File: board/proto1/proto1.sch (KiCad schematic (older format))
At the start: 86 parts, among them J1 Micro_SD_Card_Det, J10 GND, J11 J11, J11A1 J11A, J12 VBatt, J13 VBattSw, J14 LCD, J15 3.3V Out, J2 LED_DOUT, J3 Expansion, J4 +3.3V, J5 J5, J5A1 J5A, J6 J6, J6A1 J6A, J7 J7, J7A1 J7A, J8 J8, J8A1 J8A, J9 J9, J9A1 J9A, SW1 UP, SW2 LEFT, SW3 RIGHT, SW4 DOWN, SW5 ACTION, SW6 TILT, U1 MCP1603T-330I/OS

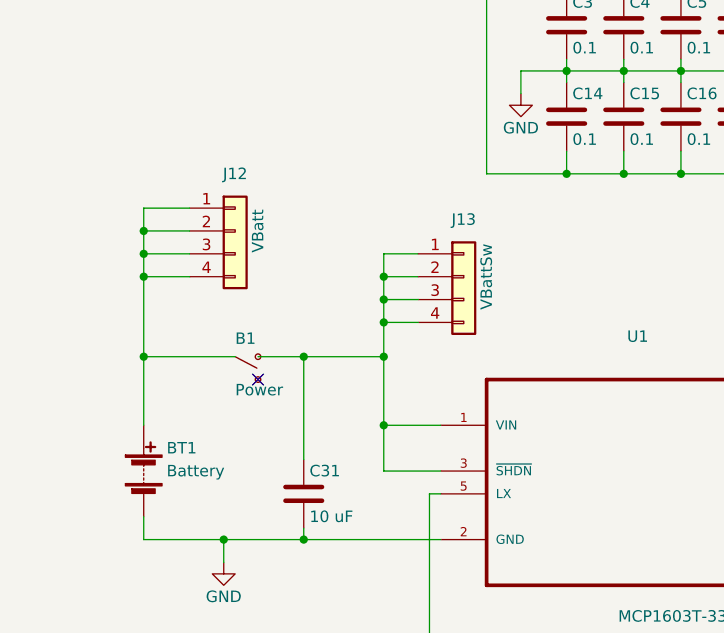
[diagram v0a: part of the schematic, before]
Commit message: layout maybe finished
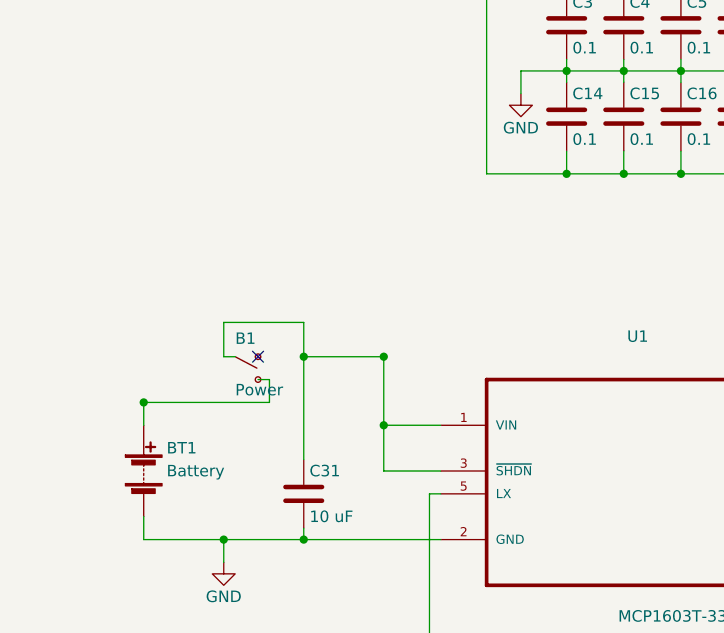
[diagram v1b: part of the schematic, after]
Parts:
- removed J12: VBatt, Pin_Headers:Pin_Header_Straight_1x04_Pitch2.54mm, symbol Conn_01x04
- removed J13: VBattSw, Pin_Headers:Pin_Header_Straight_1x04_Pitch2.54mm, symbol Conn_01x04
- J1: footprint 1140084168:1140084168 -> sdcard:newsdcard
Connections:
- net at B1.1 (B): now also BT1.1 (+)
- net at B1.2 (COM): now also C31.1, U1.1 (VIN), U1.3 (~SHDN); no longer BT1.1 (+)
- now unconnected: B1.3 (A)
